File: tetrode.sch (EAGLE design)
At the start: 34 parts, among them IC1 MEGA8-P, J1 AVR_SPI_PROG_3X2NS, U1 LM2576T-5.0/NOPB, Y1 16MHz

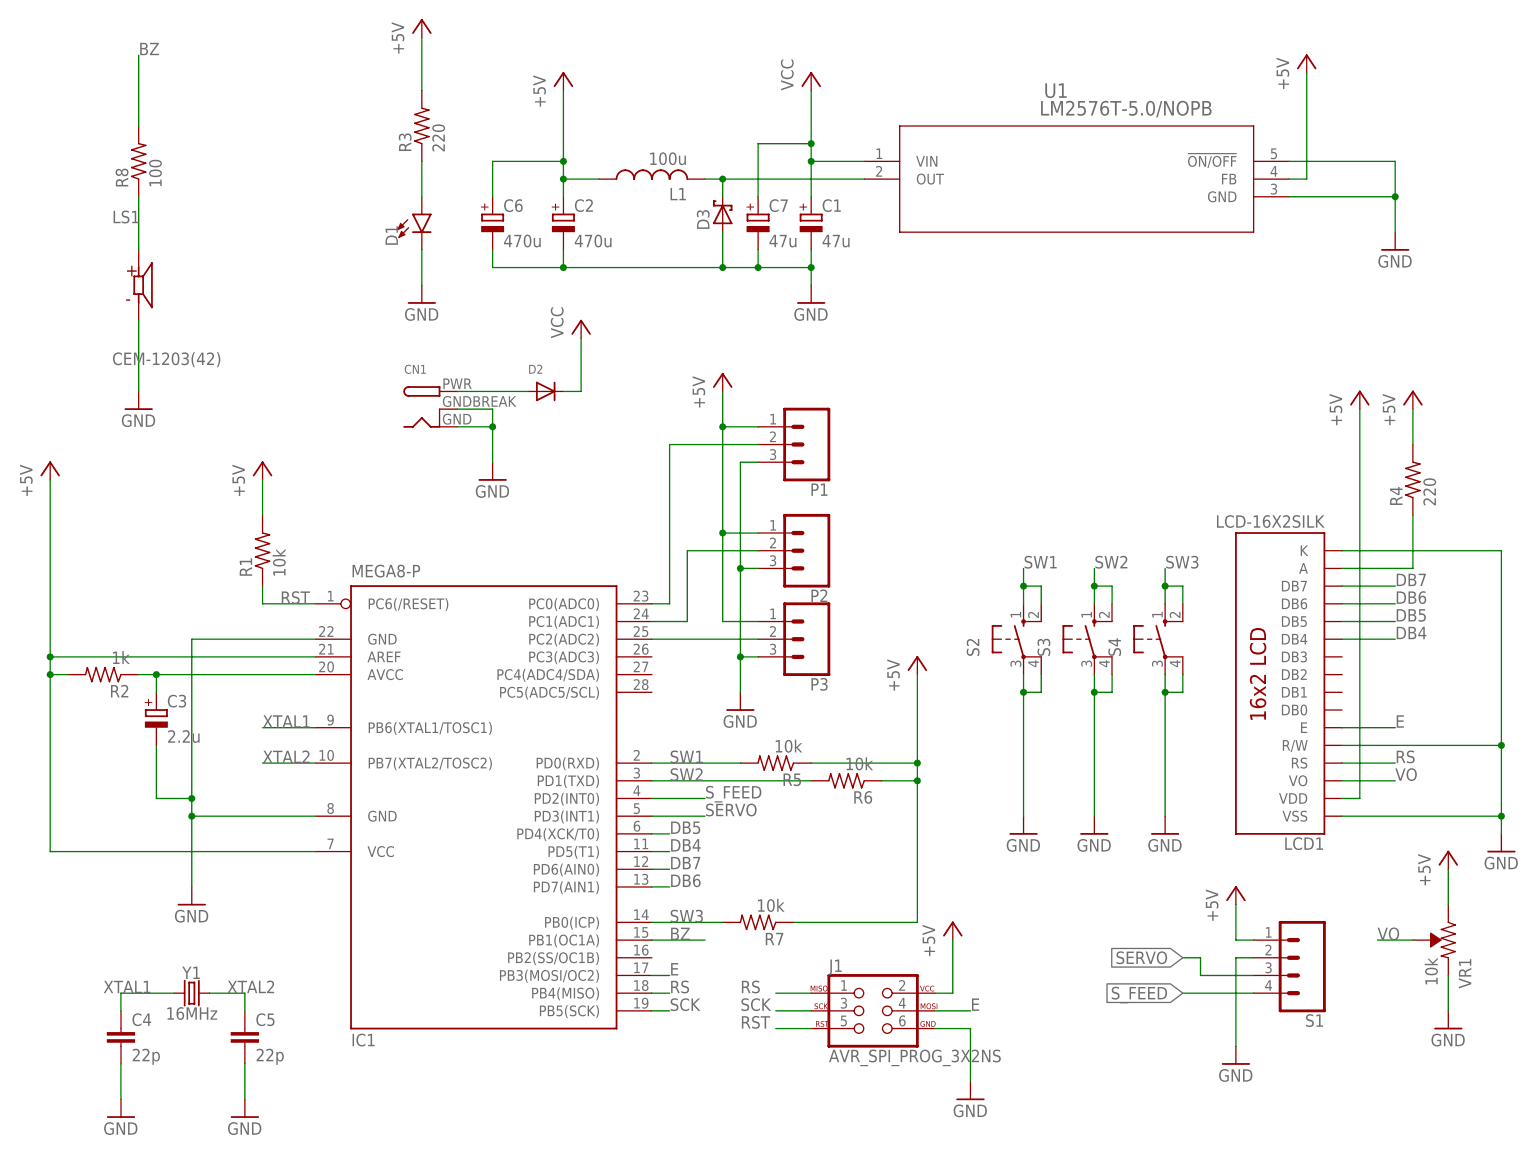
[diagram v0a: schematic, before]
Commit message: Started code
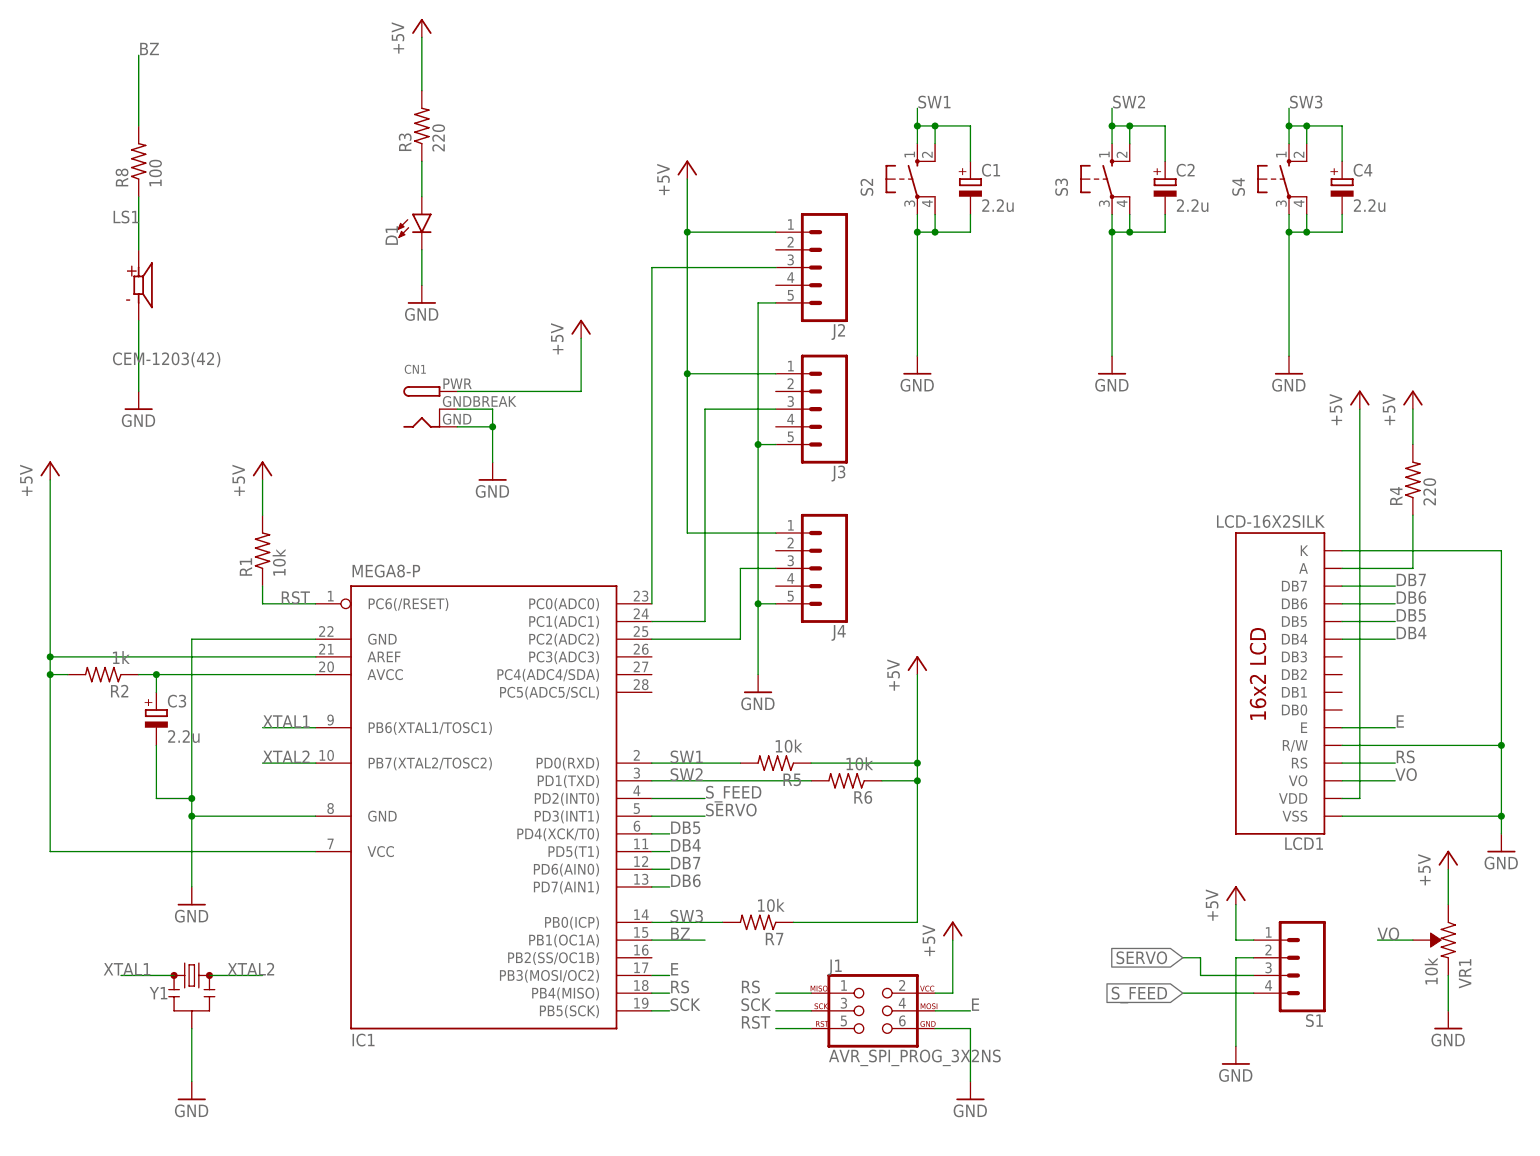
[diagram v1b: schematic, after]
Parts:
- removed C5: 22p, resistor:C-EU025-024X044
- removed C6: 470u, resistor:CPOL-EUE5-13
- removed C7: 47u, resistor:CPOL-EUE2.5-6
- removed D2: (no value), adafruit:DIODEDO-1N4148
- removed D3: (no value), adafruit:SCHOTTKY-DIODEDO201T15
- removed L1: 100u, resistor:L-US0204/5
- removed P1, P2, P3: (no value), SparkFun-Connectors:CONN_03
- removed U1: LM2576T-5.0/NOPB, LM2576T:LM2576T-5.0/NOPB
- added J2, J3, J4: (no value), SparkFun-Connectors:CONN_05
- C1: value 47u -> 2.2u; device resistor:CPOL-EUE2.5-6 -> resistor:CPOL-EUE2-5
- C2: value 470u -> 2.2u; device resistor:CPOL-EUE5-13 -> resistor:CPOL-EUE2-5
- C4: value 22p -> 2.2u; device resistor:C-EU025-024X044 -> resistor:CPOL-EUE2-5
- Y1: value 16MHz -> (none); device SparkFun-Clocks:CRYSTAL-16MHZPTH-HC49US -> SparkFun-Clocks:RESONATORPTH-7.6X3.8
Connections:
- removed net N$5: IC1.PC2(ADC2), P3.2
- removed net N$8: D3.C, L1.2, U1.OUT
- removed net VCC: C1.+, C7.+, D2.C, U1.VIN
- net +5V: now also CN1.PWR, J2.1, J3.1, J4.1; no longer C2.+, C6.+, L1.1, P1.1, P2.1, P3.1, U1.FB
- net GND: now also C4.-, J2.5, J3.5, J4.5, Y1.2; no longer C4.2, C5.2, C6.-, C7.-, D3.A, P1.3, P2.3, P3.3, U1.!ON/OFF, U1.GND
- net N$1: now also IC1.PC0(ADC0), J2.3; no longer CN1.PWR, D2.A
- net N$3: now also IC1.PC1(ADC1), J3.3; no longer IC1.PC0(ADC0), P1.2
- net N$4: now also IC1.PC2(ADC2), J4.3; no longer IC1.PC1(ADC1), P2.2
- net SW1: now also C1.+
- net SW2: now also C2.+
- net SW3: now also C4.+
- net XTAL1: no longer C4.1
- net XTAL2: now also Y1.3; no longer C5.1, Y1.2
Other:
- moved on the sheet: C1, C2, S2, S3, S4
